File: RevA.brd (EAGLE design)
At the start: 106 x 53 mm, 61 parts, among them IC1 MAX31855, IC10 DS3231/SO, IC3 MAX31855, IC4 MAX31855, IC5 MAX31855, IC9 ATMEGA32U4-AU, J1 1X2-3.5MM, J2 1X2-3.5MM, J3 1X2-3.5MM, J4 1X2-3.5MM, J5 503182-1852, U2 SPX3819-3.3, U3 MCP73831T-2ACI/OT, X1 JSTPH, X3 microUSB, Y1 8MHz

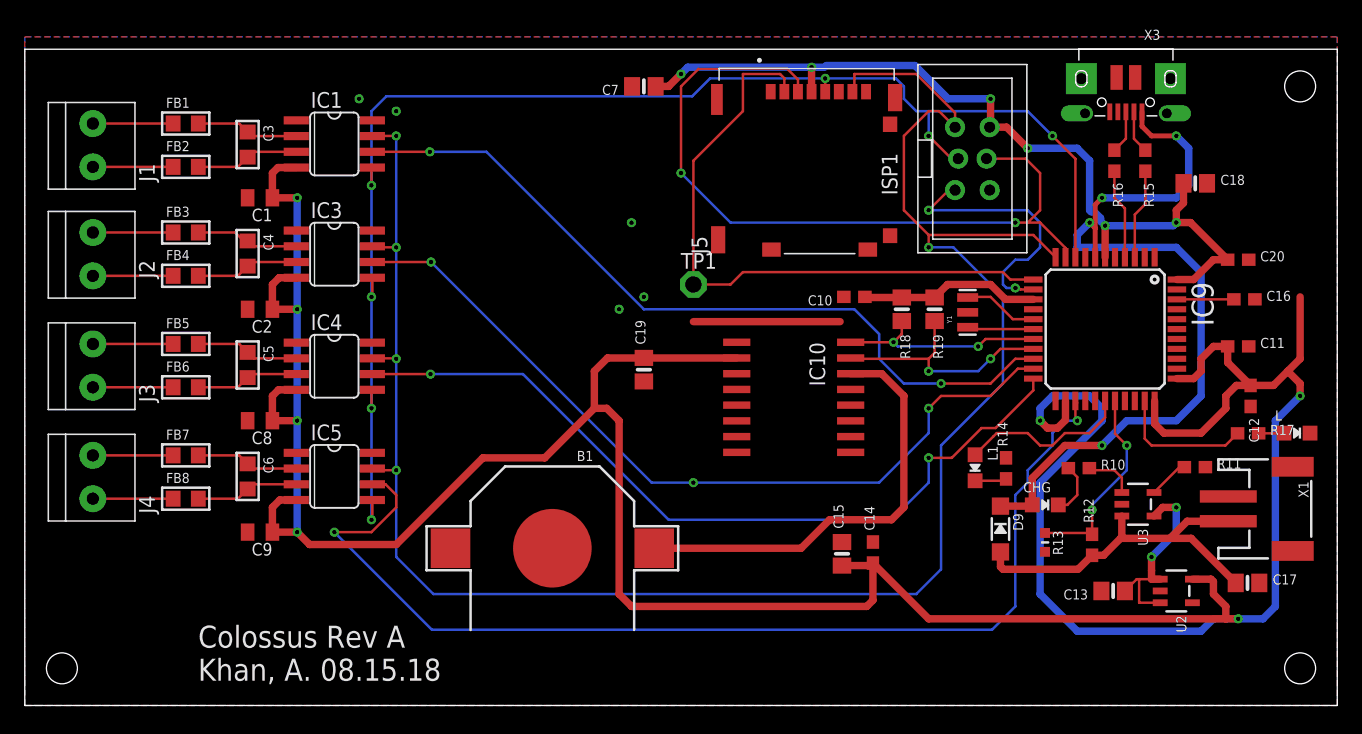
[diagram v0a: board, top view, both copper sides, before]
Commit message: Changed Layout
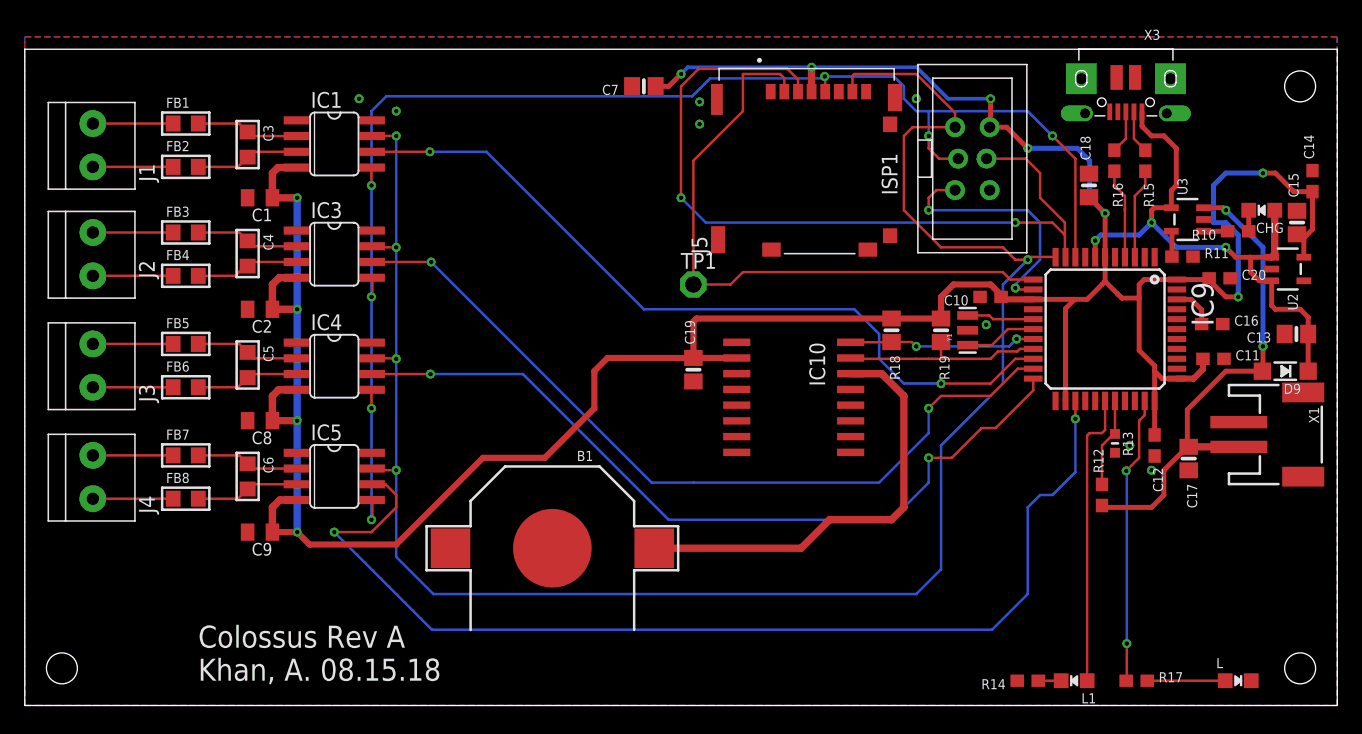
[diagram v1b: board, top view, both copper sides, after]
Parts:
- moved C14 46.5 mm to (104.0, 42.4)
- moved C15 45.5 mm to (102.8, 39.0)
- moved CHG 29.5 mm to (99.9, 40.0), turned to 90 degrees
- moved U2 27.5 mm to (102.0, 35.2)
- moved D9 26.3 mm to (101.8, 27.0), turned to 180 degrees
- moved C13 25.5 mm to (102.7, 30.0)
- moved U3 23.3 mm to (93.9, 39.2), turned to 90 degrees
- moved R10 23.1 mm to (98.0, 38.3), turned to 180 degrees
- moved R17 21.9 mm to (89.8, 2.00)
- moved L 20.6 mm to (98.0, 2.00)
- moved L1 19.0 mm to (84.8, 2.00), turned to 90 degrees
- moved R14 17.2 mm to (81.0, 2.00), turned to 180 degrees
- moved R11 17.0 mm to (93.5, 36.2)
- moved C17 11.1 mm to (94.0, 19.9), turned to 270 degrees
- moved C10 11.0 mm to (78.0, 33.0)
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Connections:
- net COIN renamed VCR
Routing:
- net +3V3: track 372.7 -> 254.6 mm, vias 13 -> 11
- net VBUS: track 81.9 -> 46.5 mm, vias 6 -> 3
- net 13: track 11.2 -> 23.3 mm, vias 0 -> 2
- net VBAT: track 29.9 -> 40.9 mm, vias 0 -> 2
- net 8: track 13.9 -> 23.8 mm
- net 9: track 16.2 -> 7.25 mm, vias 2 -> 0
- net MISO: track 158.0 -> 153.0 mm
- net N$33: track 2.62 -> 6.32 mm
- net MOSI: track 61.9 -> 65.1 mm
- net N$25: track 4.33 -> 1.70 mm
- net SDA: track 19.8 -> 17.3 mm, vias 2 -> 0
- net N$26: track 4.14 -> 1.95 mm
- net SCL: track 17.1 -> 15.1 mm
- net RST: track 21.7 -> 20.4 mm
- net N$27: track 3.30 -> 2.07 mm
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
